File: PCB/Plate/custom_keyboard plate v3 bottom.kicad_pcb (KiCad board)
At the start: 2 copper layers, 395.3 x 142.9 mm, 58 parts, among them M2 MountingHole_2.2mm_M2_ISO7380, M2.5 MountingHole_2.5mm, M3 MountingHole_3.2mm_M3

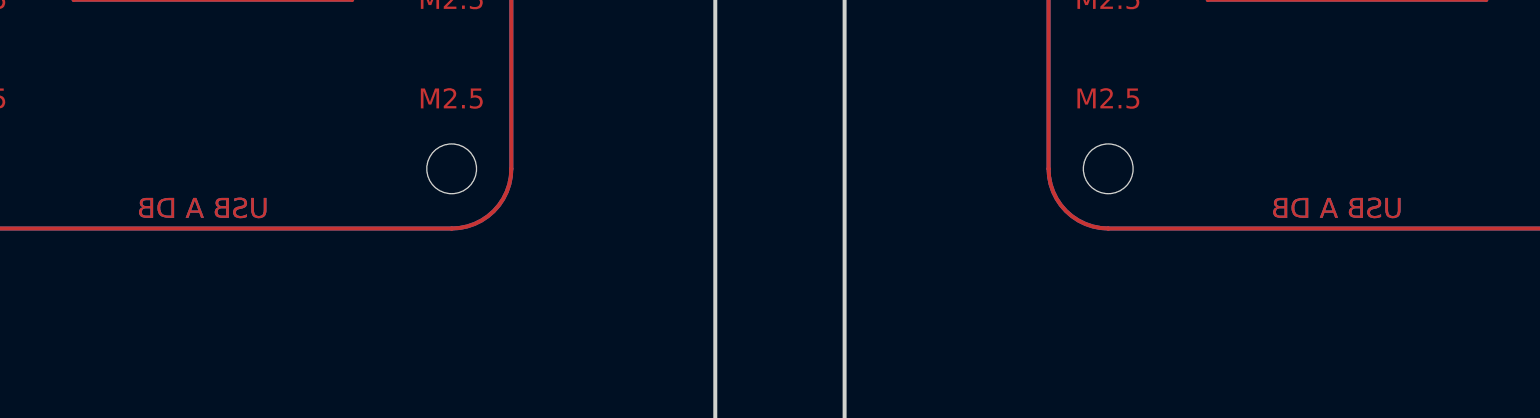
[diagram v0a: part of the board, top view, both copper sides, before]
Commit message: Final verification before ordering
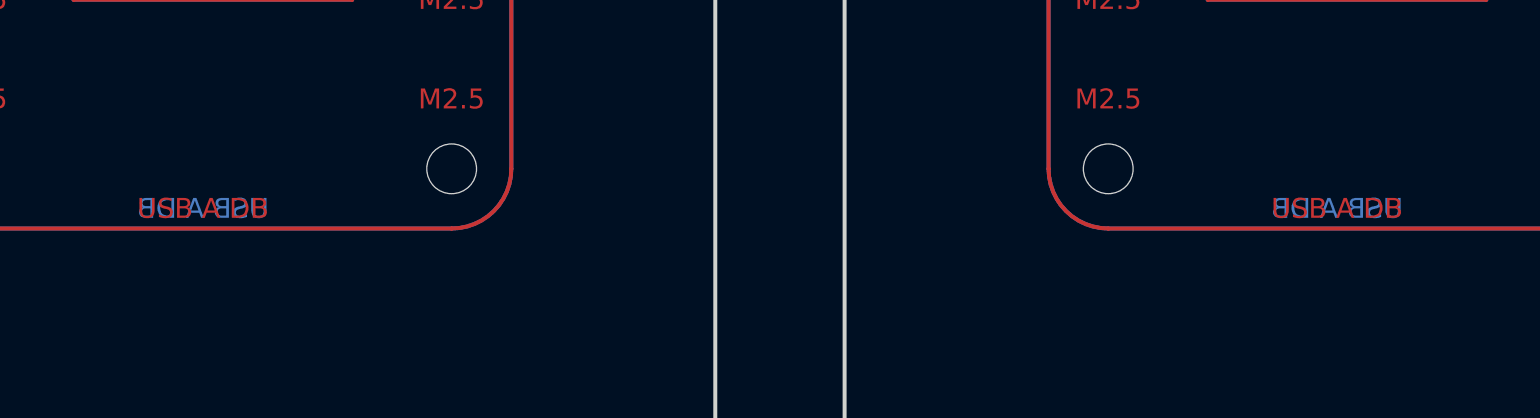
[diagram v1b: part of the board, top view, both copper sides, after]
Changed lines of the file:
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@@
   )
   (gr_text "USB A DB" (at 138.6242 97.4137) (layer "F.Cu")
-    (effects (font (size 1 1) (thickness 0.2)) (justify mirror))
+    (effects (font (size 1 1) (thickness 0.2)))
   )
   (gr_text "4 Port" (at 195.1242 98.9137 270) (layer "F.Cu")
@@
   )
   (gr_text "USB A DB" (at 81.6242 97.4137) (layer "F.Cu")
-    (effects (font (size 1 1) (thickness 0.2)) (justify mirror))
+    (effects (font (size 1 1) (thickness 0.2)))
   )
   (gr_text "USB A DB" (at 383.568499 115.6322 -90) (layer "B.Cu")
